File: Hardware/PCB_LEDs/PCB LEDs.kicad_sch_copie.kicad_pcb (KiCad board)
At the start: 2 copper layers, 33.5 x 32.5 mm, 18 parts, among them J1 Conn_01x05, U1 PCA9685PW

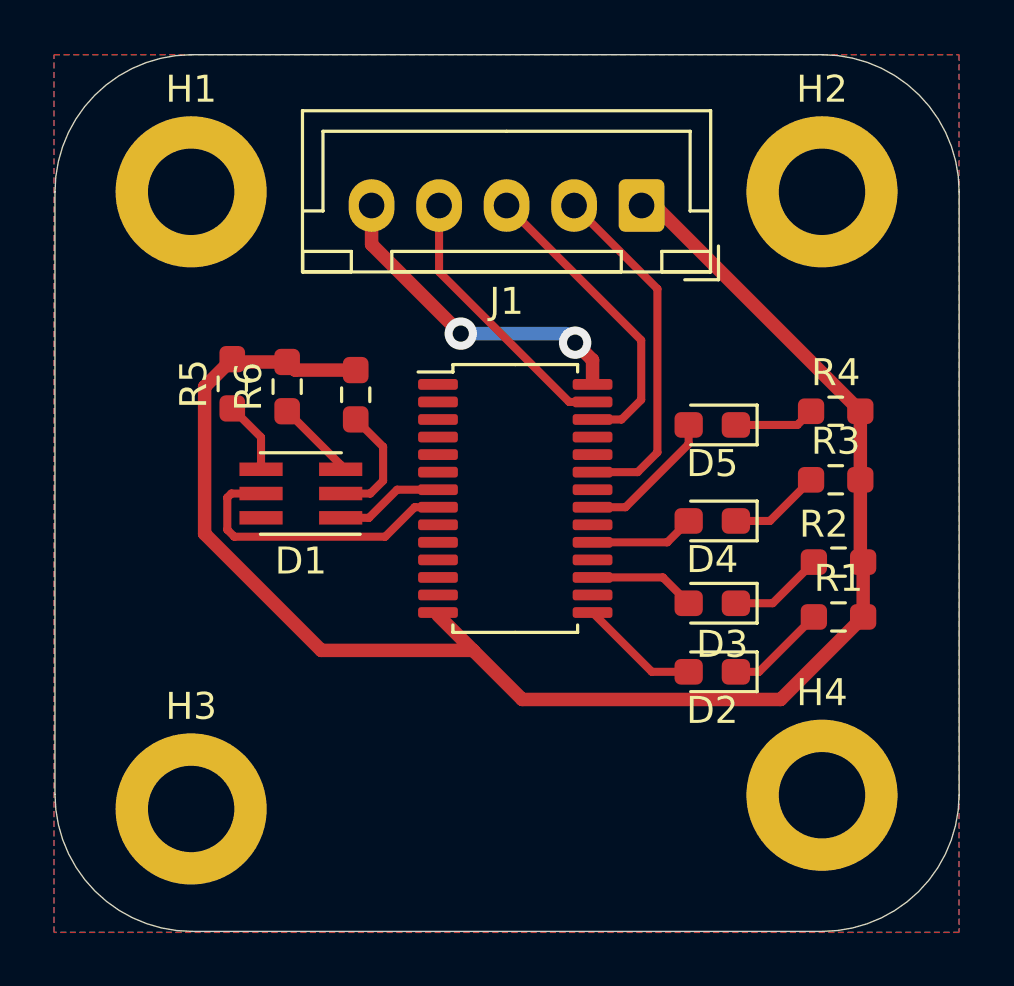
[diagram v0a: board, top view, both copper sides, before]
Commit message: PCB avec titre
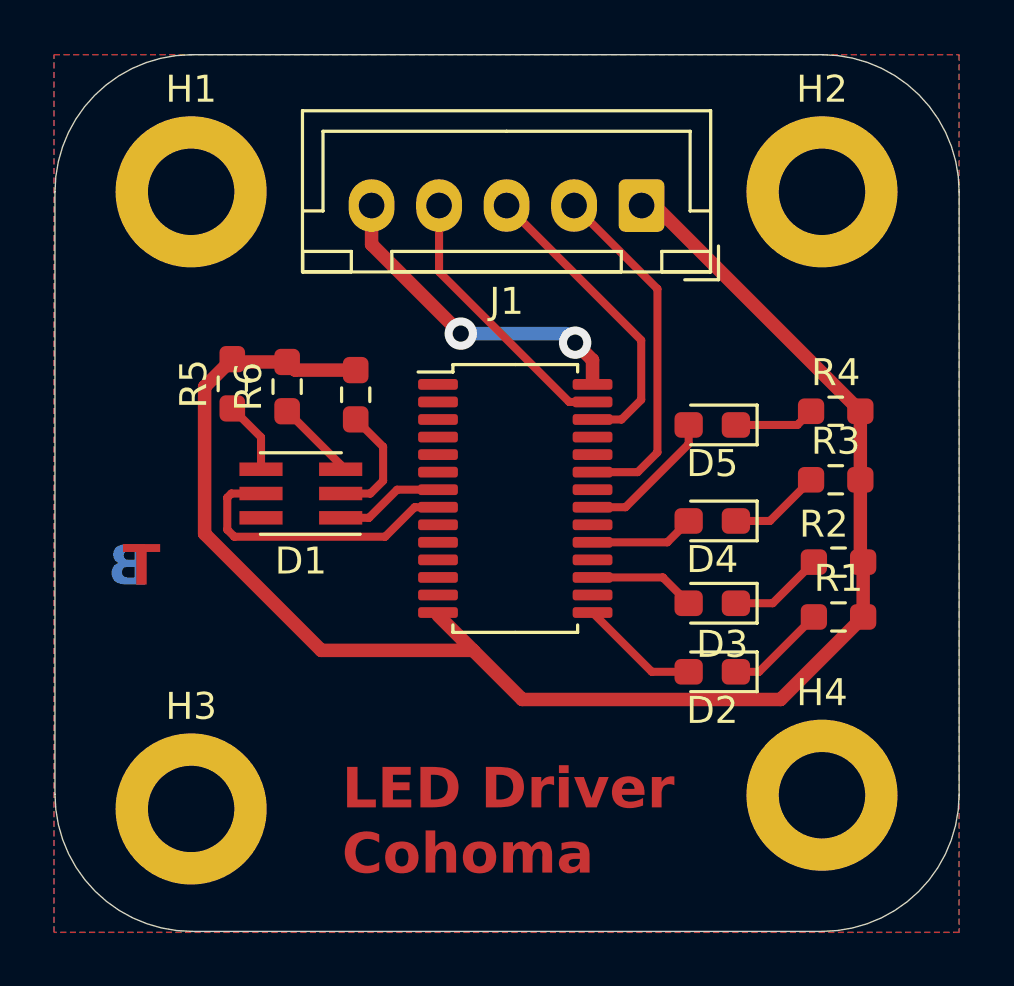
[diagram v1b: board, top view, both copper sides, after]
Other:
- board text added: "B"
- board text added: "LED Driver Cohoma"
- board text added: "T"
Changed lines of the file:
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@@
   (gr_line (start 149.86 63.5) (end 149.86 85.852)
     (stroke (width 0.05) (type default)) (layer "Edge.Cuts"))
+  (gr_text "LED Driver\nCohoma" (at 127 88.9) (layer "F.Cu")
+    (effects (font (size 1.5 1.5) (thickness 0.3) bold) (justify left bottom))
+  )
+  (gr_text "T" (at 118.872 78.232) (layer "F.Cu")
+    (effects (font (size 1.5 1.5) (thickness 0.3) bold) (justify left bottom))
+  )
+  (gr_text "B" (at 119.888 78.232) (layer "B.Cu")
+    (effects (font (size 1.5 1.5) (thickness 0.3) bold) (justify left bottom mirror))
+  )
   (dimension (type aligned) (layer "F.Cu")
     (pts (xy 121.412 57.912) (xy 144.78 57.912))

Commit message: Réparé ?
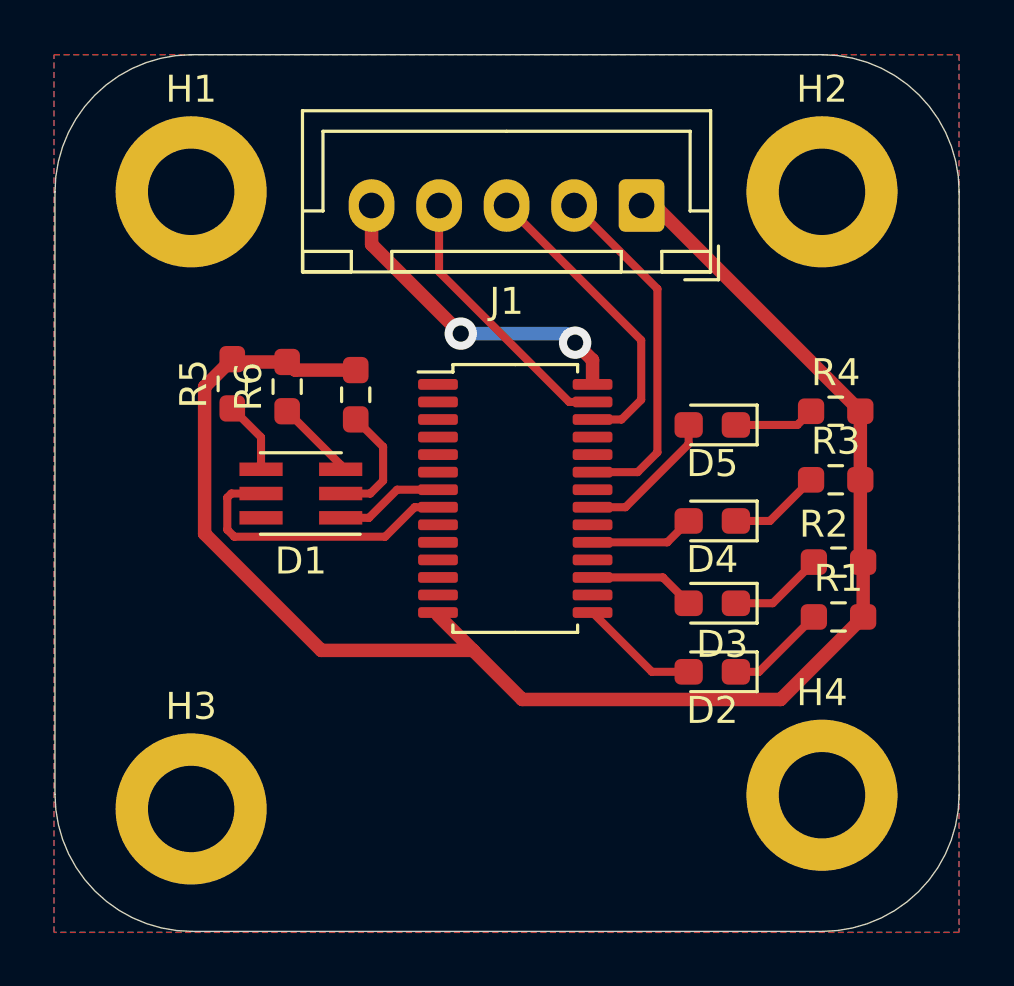
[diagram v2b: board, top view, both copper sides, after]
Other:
- board text removed: "B"
- board text removed: "LED Driver Cohoma"
- board text removed: "T"
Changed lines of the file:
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@@
   (gr_line (start 149.86 63.5) (end 149.86 85.852)
     (stroke (width 0.05) (type default)) (layer "Edge.Cuts"))
-  (gr_text "LED Driver\nCohoma" (at 127 88.9) (layer "F.Cu")
-    (effects (font (size 1.5 1.5) (thickness 0.3) bold) (justify left bottom))
-  )
-  (gr_text "T" (at 118.872 78.232) (layer "F.Cu")
-    (effects (font (size 1.5 1.5) (thickness 0.3) bold) (justify left bottom))
-  )
-  (gr_text "B" (at 119.888 78.232) (layer "B.Cu")
-    (effects (font (size 1.5 1.5) (thickness 0.3) bold) (justify left bottom mirror))
-  )
   (dimension (type aligned) (layer "F.Cu")
     (pts (xy 121.412 57.912) (xy 144.78 57.912))
